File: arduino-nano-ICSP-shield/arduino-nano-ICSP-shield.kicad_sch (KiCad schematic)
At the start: 11 parts, among them J1 Analog, J2 Digital, J3 AVR-ISP-6, J4 Conn_02x04_Counter_Clockwise

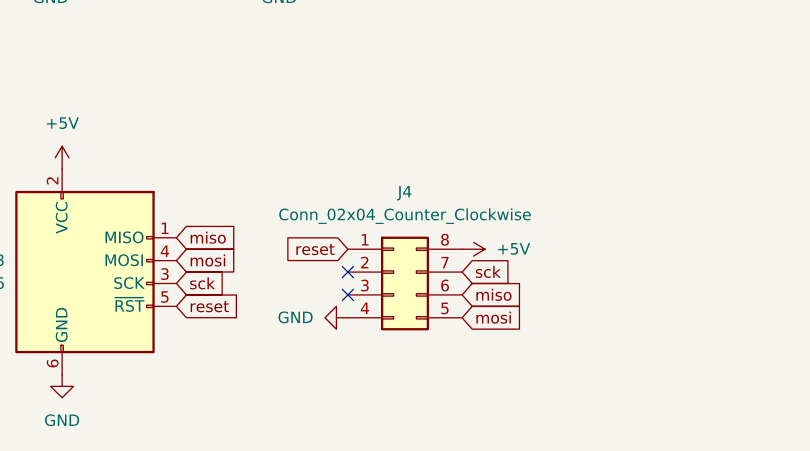
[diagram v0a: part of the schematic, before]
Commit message: improv
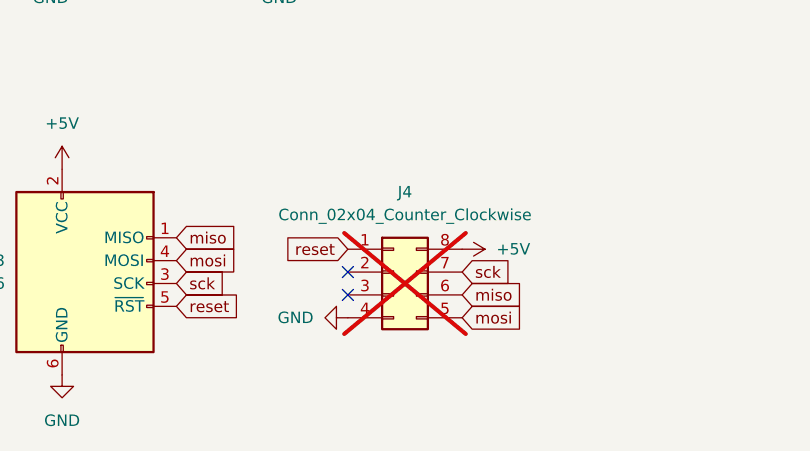
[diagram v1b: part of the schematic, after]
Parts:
- J4: now not fitted; now left out of the parts list
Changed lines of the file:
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@@
 		(at 71.12 99.06 0)
 		(unit 1)
-		(exclude_from_sim no)
-		(in_bom yes)
-		(on_board yes)
-		(dnp no)
+		(exclude_from_sim yes)
+		(in_bom no)
+		(on_board no)
+		(dnp yes)
 		(fields_autoplaced yes)
 		(property "Reference" "J4"

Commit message: Readd Clip
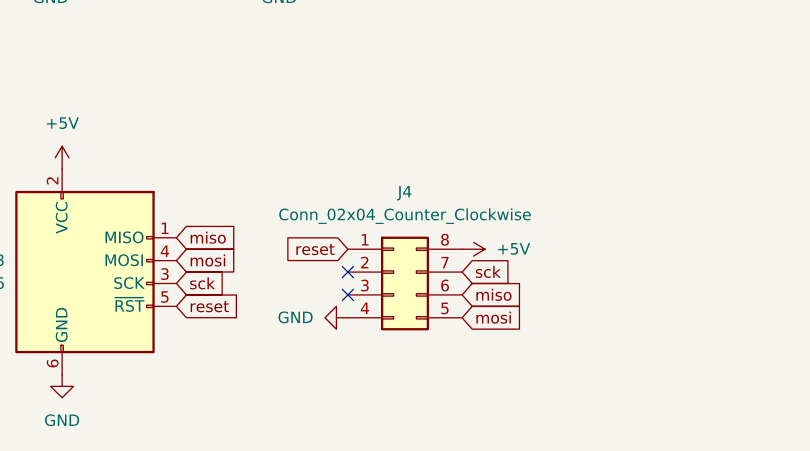
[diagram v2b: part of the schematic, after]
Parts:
- J4: now fitted; now in the parts list
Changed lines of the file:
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@@
 		(at 71.12 99.06 0)
 		(unit 1)
-		(exclude_from_sim yes)
-		(in_bom no)
-		(on_board no)
-		(dnp yes)
+		(exclude_from_sim no)
+		(in_bom yes)
+		(on_board yes)
+		(dnp no)
 		(fields_autoplaced yes)
 		(property "Reference" "J4"
